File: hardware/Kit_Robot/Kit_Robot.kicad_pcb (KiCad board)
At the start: 2 copper layers, 48.9 x 49.2 mm, 12 parts, among them Q3 BC548, Q4 BC548, SW2 On

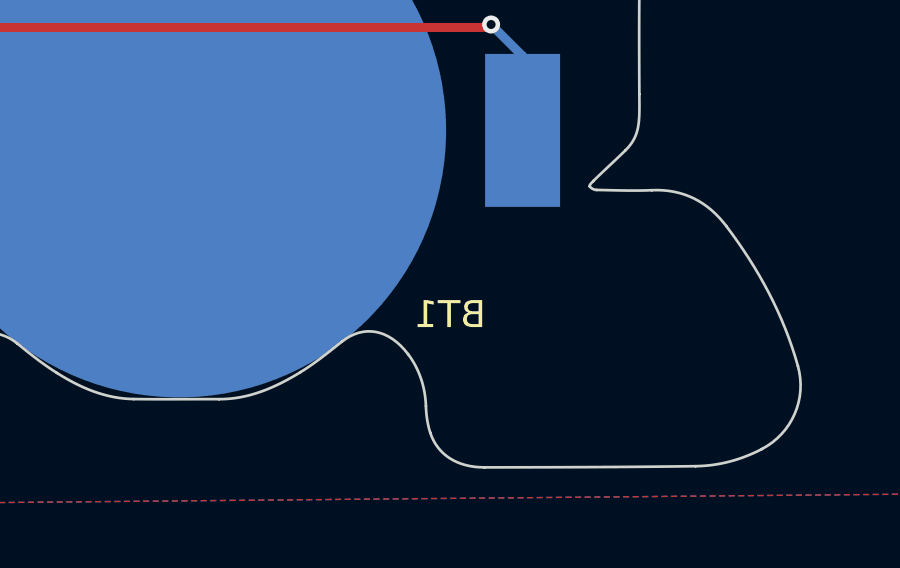
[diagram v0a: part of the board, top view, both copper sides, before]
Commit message: feat(hw):Labels_Updated
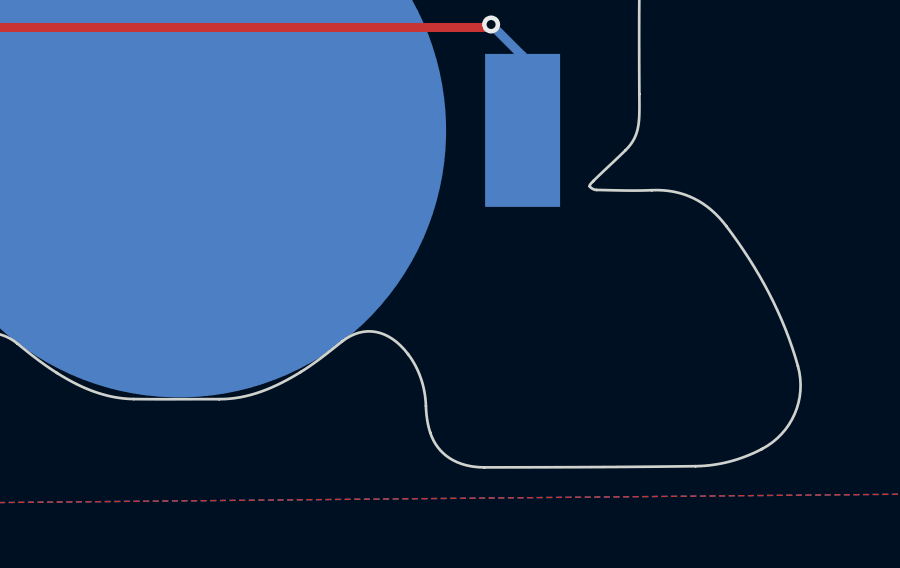
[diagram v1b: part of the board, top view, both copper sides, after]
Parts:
- added kibuzzard-6AC42980: G***, kibuzzard-6AC42980, B.Cu at (126.0, 28.1)
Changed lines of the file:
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@@
 		)
+	)
+	(footprint "kibuzzard-6AC42980"
+		(layer "B.Cu")
+		(at 126.04 28.08 180)
+		(descr "Generated with KiBuzzard")
+		(tags "kb_params=eyJBbGlnbm1lbnRDaG9pY2UiOiAiQ2VudGVyIiwgIkNhcExlZnRDaG9pY2UiOiAiPCIsICJDYXBSaWdodENob2ljZSI6ICI8IiwgIkZvbnRDb21ib0JveCI6ICJVYnVudHVNb25vLUIiLCAiSGVpZ2h0Q3RybCI6IDAuOCwgIkxheWVyQ29tYm9Cb3giOiAiRi5TaWxrUyIsICJMaW5lU3BhY2luZ0N0cmwiOiAwLjcsICJNdWx0aUxpbmVUZXh0IjogIk9OIiwgIlBhZGRpbmdCb3R0b21DdHJsIjogNS4wLCAiUGFkZGluZ0xlZnRDdHJsIjogNS4wLCAiUGFkZGluZ1JpZ2h0Q3RybCI6IDUuMCwgIlBhZGRpbmdUb3BDdHJsIjogNS4wLCAiV2lkdGhDdHJsIjogMC44LCAiYWR2YW5jZWRDaGVja2JveCI6IGZhbHNlLCAiaW5saW5lRm9ybWF0VGV4dGJveCI6IGZhbHNlLCAibGluZW92ZXJTdHlsZUNob2ljZSI6ICJTcXVhcmUiLCAibGluZW92ZXJUaGlja25lc3NDdHJsIjogMX0=")
+		(property "Reference" "kibuzzard-6AC42980"
+			(at 0 4.00395 0)
+			(layer "B.SilkS")
+			(hide yes)
+			(effects
+				(font
+					(size 0.001 0.001)
+				)
+				(justify mirror)
+			)
+		)
+		(property "Value" "G***"
+			(at 0 -4.00395 0)
+			(layer "B.SilkS")
+			(hide yes)
+			(effects
+				(font
+					(size 0.001 0.001)
+				)
+				(justify mirror)
+			)
+		)
+		(property "Datasheet" ""
+			(at 0 0 0)
+			(layer "B.Fab")
+			(hide yes)
+			(effects
+				(font
+					(size 1.27 1.27)
+				)
+				(justify mirror)
+			)
+		)
+		(property "Description" ""
+			(at 0 0 0)
+			(layer "B.Fab")
+			(hide yes)
+			(effects
+				(font
+					(size 1.27 1.27)
+				)
+				(justify mirror)
+			)
+		)
+		(attr board_only exclude_from_pos_files exclude_from_bom)
+		(duplicate_pad_numbers_are_jumpers no)
+		(fp_poly
+			(pts
+				(xy -0.43748 0) (xy -0.436349 -0.056381) (xy -0.432956 -0.109208) (xy -0.414863 -0.197738) (xy -0.376737 -0.257189)
+				(xy -0.310824 -0.27916) (xy -0.245557 -0.257189) (xy -0.206785 -0.197092) (xy -0.188691 -0.108562)
+				(xy -0.185299 -0.05622) (xy -0.184168 0) (xy -0.185299 0.056381) (xy -0.188691 0.109208) (xy -0.206785 0.197738)
+				(xy -0.244911 0.257189) (xy -0.310824 0.27916) (xy -0.376737 0.257189) (xy -0.414863 0.197092) (xy -0.432956 0.108562)
+				(xy -0.436349 0.05622) (xy -0.43748 0)
+			)
+			(stroke
+				(width 0)
+				(type solid)
+			)
+			(fill yes)
+			(layer "B.SilkS")
+		)
+		(fp_poly
+			(pts
+				(xy -0.599031 0.95595) (xy -1.137534 0.95595) (xy -1.774834 0) (xy -1.137534 -0.95595) (xy -0.599031 -0.95595)
+				(xy -0.309532 -0.95595) (xy -0.309532 -0.417447) (xy -0.396051 -0.405744) (xy -0.46778 -0.370634)
+				(xy -0.524717 -0.312116) (xy -0.557229 -0.25311) (xy -0.580452 -0.181422) (xy -0.594386 -0.097052)
+				(xy -0.599031 0) (xy -0.594265 0.097052) (xy -0.579968 0.181422) (xy -0.556139 0.25311) (xy -0.522779 0.312116)
+				(xy -0.465338 0.370634) (xy -0.394687 0.405744) (xy -0.310824 0.417447) (xy -0.224376 0.405744)
+				(xy -0.152863 0.370634) (xy -0.096284 0.312116) (xy -0.064055 0.25311) (xy -0.041034 0.181422) (xy -0.027221 0.097052)
+				(xy -0.022617 0) (xy -0.027302 -0.097052) (xy -0.041357 -0.181422) (xy -0.064782 -0.25311) (xy -0.097577 -0.312116)
+				(xy -0.154443 -0.370634) (xy -0.225094 -0.405744) (xy -0.309532 -0.417447) (xy -0.309532 -0.95595)
+				(xy 0.471082 -0.95595) (xy 0.471082 -0.400646) (xy 0.433818 -0.311973) (xy 0.3944 -0.223443) (xy 0.352827 -0.135057)
+				(xy 0.309101 -0.04667) (xy 0.26322 0.04186) (xy 0.215186 0.130533) (xy 0.215186 -0.400646) (xy 0.071729 -0.400646)
+				(xy 0.071729 0.399354) (xy 0.199677 0.399354) (xy 0.235864 0.340065) (xy 0.272052 0.275929) (xy 0.307754 0.209532)
+				(xy 0.342488 0.143457) (xy 0.375444 0.078514) (xy 0.405816 0.015509) (xy 0.432795 -0.042649) (xy 0.455574 -0.093053)
+				(xy 0.455574 0.399354) (xy 0.599031 0.399354) (xy 0.599031 -0.400646) (xy 0.471082 -0.400646) (xy 0.471082 -0.95595)
+				(xy 0.599031 -0.95595) (xy 1.137534 -0.95595) (xy 1.774834 -0.95595) (xy 1.137534 0) (xy 1.774834 0.95595)
+				(xy 1.137534 0.95595) (xy 0.599031 0.95595) (xy -0.599031 0.95595)
+			)
+			(stroke
+				(width 0)
+				(type solid)
+			)
+			(fill yes)
+			(layer "B.SilkS")
+		)
+		(embedded_fonts no)
 	)
 	(footprint "Button_Switch_SMD:SW_SPDT_Shouhan_MSK12C02"
@@
 		(at 116.65 60.14 180)
 		(property "Reference" "BT1"
-			(at -9.03 -6.14 0)
-			(layer "F.SilkS")
+			(at -9.03 -6.14 -0)
+			(layer "B.SilkS")
 			(effects
 				(font
@@
 					(thickness 0.15)
 				)
-				(justify mirror)
-			)
-		)
+			)
+		)

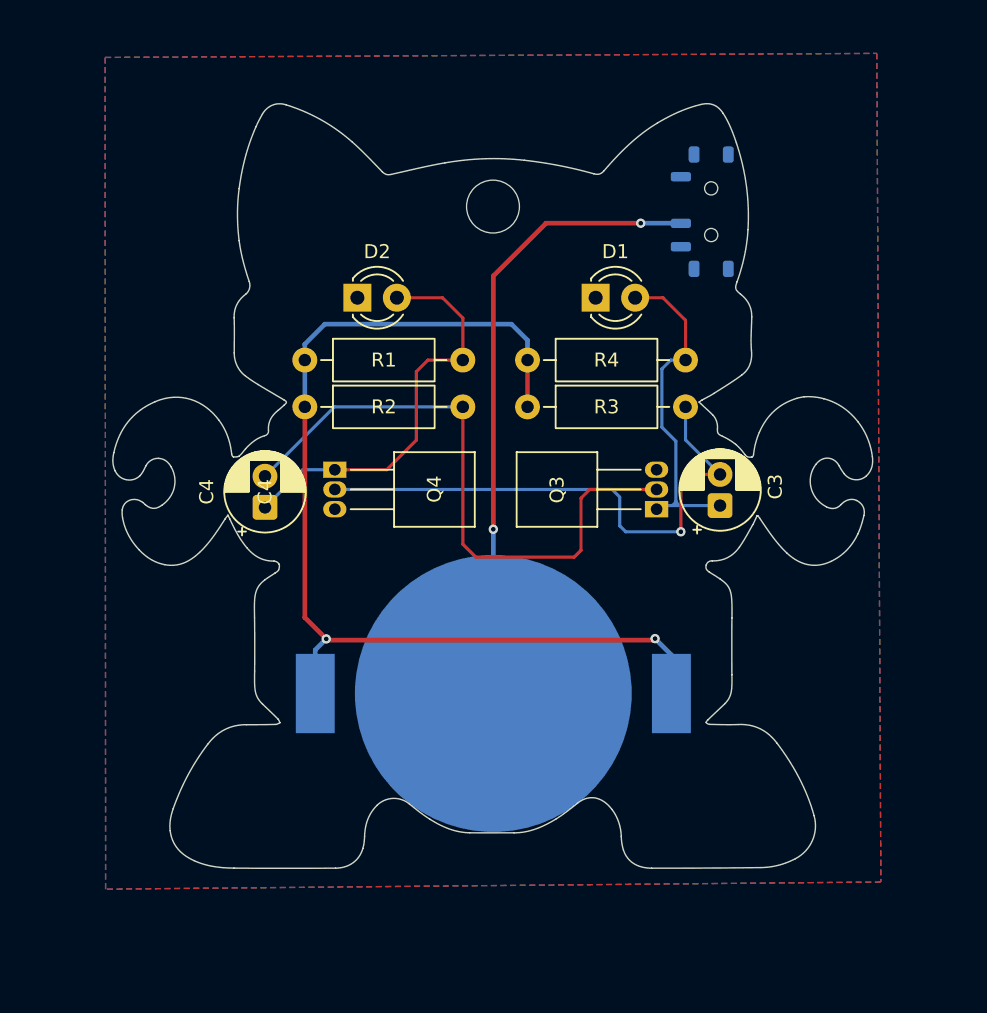
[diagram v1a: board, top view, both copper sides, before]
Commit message: feat(Hw):Projects_Added
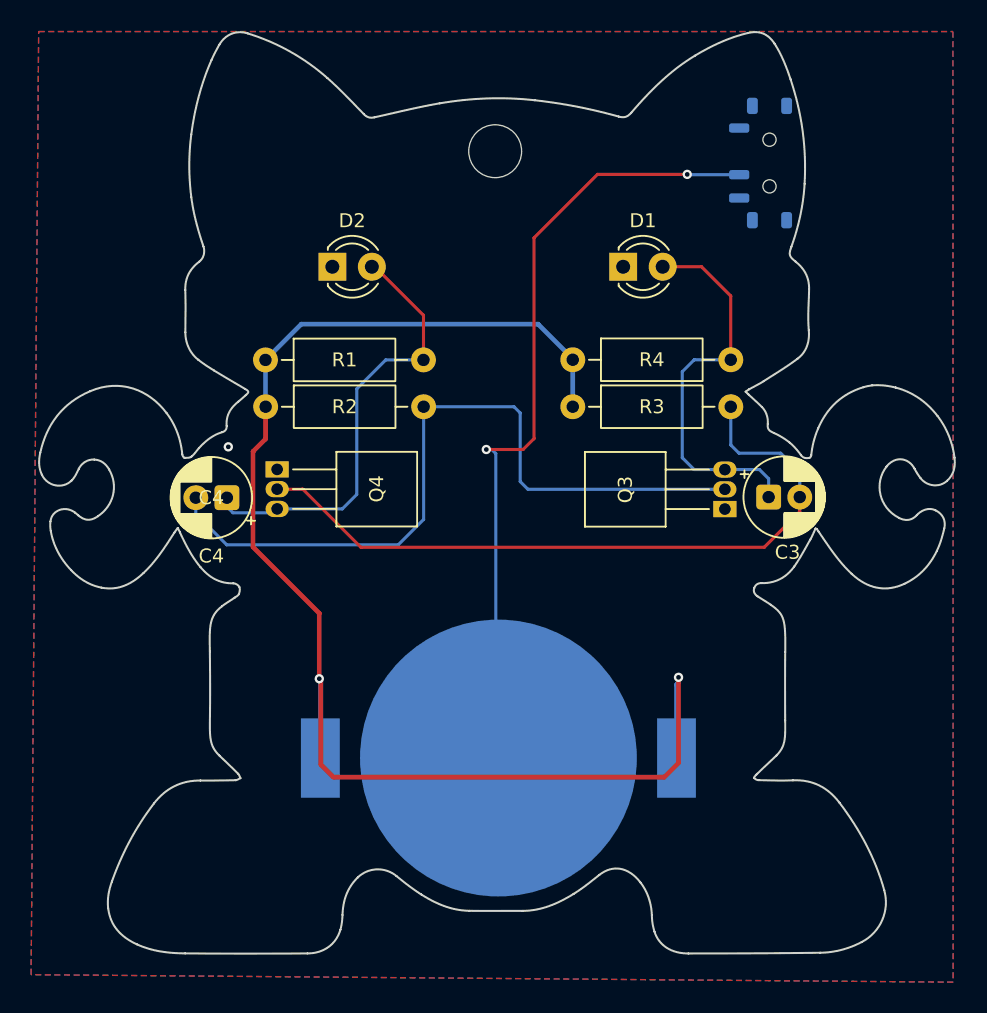
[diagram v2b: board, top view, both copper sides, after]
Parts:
- moved SW2 4.88 mm to (134.4, 26.0)
- moved Q3 4.39 mm to (131.5, 48.3)
- moved BT1 4.16 mm to (117.0, 64.3)
- moved Q4 3.71 mm to (102.8, 45.7)
- moved kibuzzard-6AC42980 3.31 mm to (129.3, 27.8)
- moved C3 3.17 mm to (134.4, 47.5), turned to 0 degrees
- moved R4 2.91 mm to (121.8, 38.7)
- moved R3 2.91 mm to (121.8, 41.7)
- moved D1 2.66 mm to (125.0, 32.7)
- moved D2 2.56 mm to (106.3, 32.7)
- moved R1 2.53 mm to (102.0, 38.7)
- moved C4 2.53 mm to (99.5, 47.5), turned to 180 degrees
- moved R2 2.52 mm to (102.0, 41.7)
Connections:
- Q3 pad 1: Net-(D1-A) -> GND
- Q3 pad 3: GND -> Net-(D1-A)
- Q4 pad 1: Net-(D2-A) -> GND
- Q4 pad 3: GND -> Net-(D2-A)
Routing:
- net +3.3V: track 68.1 -> 92.5 mm
- net Net-(BT1--): track 40.3 -> 51.5 mm
- net Net-(Q4-B): track 35.6 -> 46.3 mm, vias 1 -> 0
- net Net-(Q3-B): track 40.0 -> 48.6 mm
- net Net-(D1-A): track 22.1 -> 25.5 mm
- net Net-(D2-A): track 26.7 -> 28.9 mm
- net GND: vias 0 -> 1
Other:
- board size 48.9 x 49.2 mm -> 58.9 x 59.3 mm
